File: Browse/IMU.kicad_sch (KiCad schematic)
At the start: 2 parts

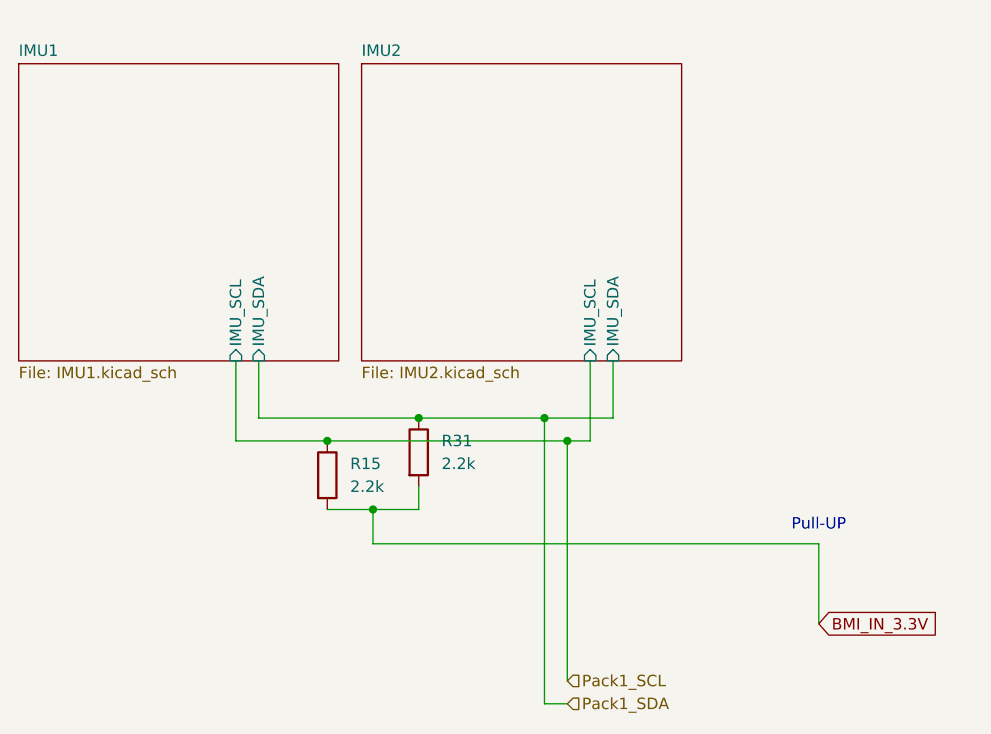
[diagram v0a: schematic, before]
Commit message: Deploying to gh-pages from @ Nautilus-UUV/nautilus-mainboard-PCB@a81f7ffbfc5f9b51f47d7f388c30fcea2673b9ea 🚀
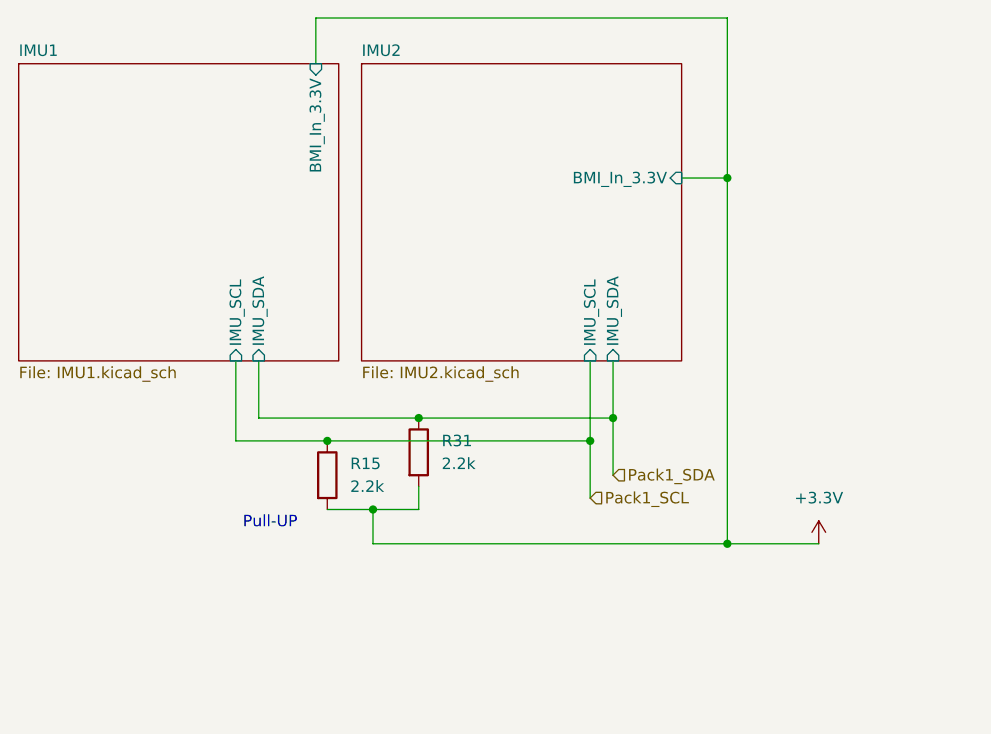
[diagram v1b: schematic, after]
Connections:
- net BMI_IN_3.3V renamed +3.3V
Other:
- sheet IMU1 ports: added BMI_In_3.3V; removed none
- sheet IMU2 ports: added BMI_In_3.3V; removed none
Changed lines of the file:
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@@
 (kicad_sch (version 20250114) (generator "eeschema") (generator_version "9.0")
   (paper "A4")
+  (junction (at 127 95.25) (diameter 0) (color 0 0 0 0)
+  )
   (junction (at 102.87 102.87) (diameter 0) (color 0 0 0 0)
   )
+  (junction (at 142.24 66.04) (diameter 0) (color 0 0 0 0)
+  )
   (junction (at 97.79 95.25) (diameter 0) (color 0 0 0 0)
   )
-  (junction (at 124.46 95.25) (diameter 0) (color 0 0 0 0)
+  (junction (at 129.54 92.71) (diameter 0) (color 0 0 0 0)
+  )
+  (junction (at 142.24 106.68) (diameter 0) (color 0 0 0 0)
   )
   (junction (at 107.95 92.71) (diameter 0) (color 0 0 0 0)
   )
-  (junction (at 121.92 92.71) (diameter 0) (color 0 0 0 0)
-  )
-  (wire (pts (xy 124.46 124.46) (xy 121.92 124.46))
-    (stroke (width 0) (type default))
-  )
-  (wire (pts (xy 124.46 95.25) (xy 124.46 121.92))
+  (wire (pts (xy 142.24 66.04) (xy 142.24 106.68))
+    (stroke (width 0) (type default))
+  )
+  (wire (pts (xy 96.52 48.26) (xy 142.24 48.26))
+    (stroke (width 0) (type default))
+  )
+  (wire (pts (xy 127 95.25) (xy 127 101.6))
     (stroke (width 0) (type default))
   )
@@
     (stroke (width 0) (type default))
   )
-  (wire (pts (xy 127 95.25) (xy 124.46 95.25))
-    (stroke (width 0) (type default))
-  )
-  (wire (pts (xy 152.4 115.57) (xy 152.4 106.68))
-    (stroke (width 0) (type default))
-  )
   (wire (pts (xy 97.79 95.25) (xy 87.63 95.25))
     (stroke (width 0) (type default))
   )
-  (wire (pts (xy 124.46 95.25) (xy 97.79 95.25))
+  (wire (pts (xy 97.79 95.25) (xy 127 95.25))
     (stroke (width 0) (type default))
   )
@@
     (stroke (width 0) (type default))
   )
-  (wire (pts (xy 107.95 92.71) (xy 121.92 92.71))
+  (wire (pts (xy 107.95 92.71) (xy 129.54 92.71))
+    (stroke (width 0) (type default))
+  )
+  (wire (pts (xy 142.24 66.04) (xy 137.16 66.04))
+    (stroke (width 0) (type default))
+  )
+  (wire (pts (xy 142.24 106.68) (xy 102.87 106.68))
     (stroke (width 0) (type default))
   )
@@
     (stroke (width 0) (type default))
   )
+  (wire (pts (xy 96.52 53.34) (xy 96.52 48.26))
+    (stroke (width 0) (type default))
+  )
   (wire (pts (xy 107.95 100.33) (xy 107.95 102.87))
     (stroke (width 0) (type default))
   )
-  (wire (pts (xy 121.92 92.71) (xy 121.92 124.46))
+  (wire (pts (xy 129.54 92.71) (xy 129.54 99.06))
+    (stroke (width 0) (type default))
+  )
+  (wire (pts (xy 142.24 48.26) (xy 142.24 66.04))
     (stroke (width 0) (type default))
   )
@@
     (stroke (width 0) (type default))
   )
-  (wire (pts (xy 152.4 106.68) (xy 102.87 106.68))
-    (stroke (width 0) (type default))
-  )
-  (wire (pts (xy 121.92 92.71) (xy 129.54 92.71))
-    (stroke (width 0) (type default))
-  )
-  (text "Pull-UP" (exclude_from_sim no) (at 152.4 104.648 0)
+  (wire (pts (xy 152.4 106.68) (xy 142.24 106.68))
+    (stroke (width 0) (type default))
+  )
+  (text "Pull-UP" (exclude_from_sim no) (at 91.44 104.394 0)
     (effects (font (size 1.27 1.27)))
   )
-  (global_label "BMI_IN_3.3V" (shape input) (at 152.4 115.57 0) (fields_autoplaced)
+  (hierarchical_label "Pack1_SDA" (shape input) (at 129.54 99.06 0)
     (effects (font (size 1.27 1.27)) (justify left))
-    (property "Intersheetrefs" "${INTERSHEET_REFS}" (at 166.6943 115.57 0)
-      (effects (font (size 1.27 1.27)) (justify left) (hide yes))
-    )
-  )
-  (hierarchical_label "Pack1_SDA" (shape input) (at 124.46 124.46 0)
-    (effects (font (size 1.27 1.27)) (justify left))
-  )
-  (hierarchical_label "Pack1_SCL" (shape input) (at 124.46 121.92 0)
+  )
+  (hierarchical_label "Pack1_SCL" (shape input) (at 127 101.6 0)
     (effects (font (size 1.27 1.27)) (justify left))
   )
@@
         (path "/ce1819b2-f280-40ed-834f-6fe4d12f809d/bdf8f7d6-a5ee-4741-925d-5019e8cbdfce"
           (reference "R15") (unit 1)
+        )
+      )
+    )
+  )
+  (symbol (lib_id "power:+3.3V") (at 152.4 106.68 0) (unit 1)
+    (exclude_from_sim no) (in_bom yes) (on_board yes) (dnp no) (fields_autoplaced)
+    (property "Reference" "#PWR033" (at 152.4 110.49 0)
+      (effects (font (size 1.27 1.27)) (hide yes))
+    )
+    (property "Value" "+3.3V" (at 152.4 101.6 0)
+      (effects (font (size 1.27 1.27)))
+    )
+    (property "Footprint" "" (at 152.4 106.68 0)
+      (effects (font (size 1.27 1.27)) (hide yes))
+    )
+    (property "Datasheet" "" (at 152.4 106.68 0)
+      (effects (font (size 1.27 1.27)) (hide yes))
+    )
+    (property "Description" "Power symbol creates a global label with name \"+3.3V\"" (at 152.4 106.68 0)
+      (effects (font (size 1.27 1.27)) (hide yes))
+    )
+    (pin "1")
+    (instances
+      (project ""
+        (path "/ce1819b2-f280-40ed-834f-6fe4d12f809d/bdf8f7d6-a5ee-4741-925d-5019e8cbdfce"
+          (reference "#PWR033") (unit 1)
         )
       )
@@
       (effects (font (size 1.27 1.27)) (justify left))
     )
+    (pin "BMI_In_3.3V" input (at 96.52 53.34 90)
+      (effects (font (size 1.27 1.27)) (justify right))
+    )
     (instances
       (project "nautilus_mainboard"
@@
       (effects (font (size 1.27 1.27)) (justify left))
     )
-    (instances
+    (pin "BMI_In_3.3V" input (at 137.16 66.04 0)
+      (effects (font (size 1.27 1.27)) (justify right))
+    )
+    (instances
